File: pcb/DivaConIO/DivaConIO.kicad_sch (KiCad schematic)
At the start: 59 parts, among them J1 Conn_01x06_MountingPin, J2 Conn_01x04_MountingPin, J3 Conn_01x06_MountingPin, J4 Conn_01x08_MountingPin, J5 JST_SH_BM03B-SRSS-TB, J6 Conn_01x05_MountingPin, J7 Conn_01x06_MountingPin, Q1 BSS138, Q2 BSS138, Q3 BSS138, Q4 BSS138, Q5 BSS138, SW1 SW_Push

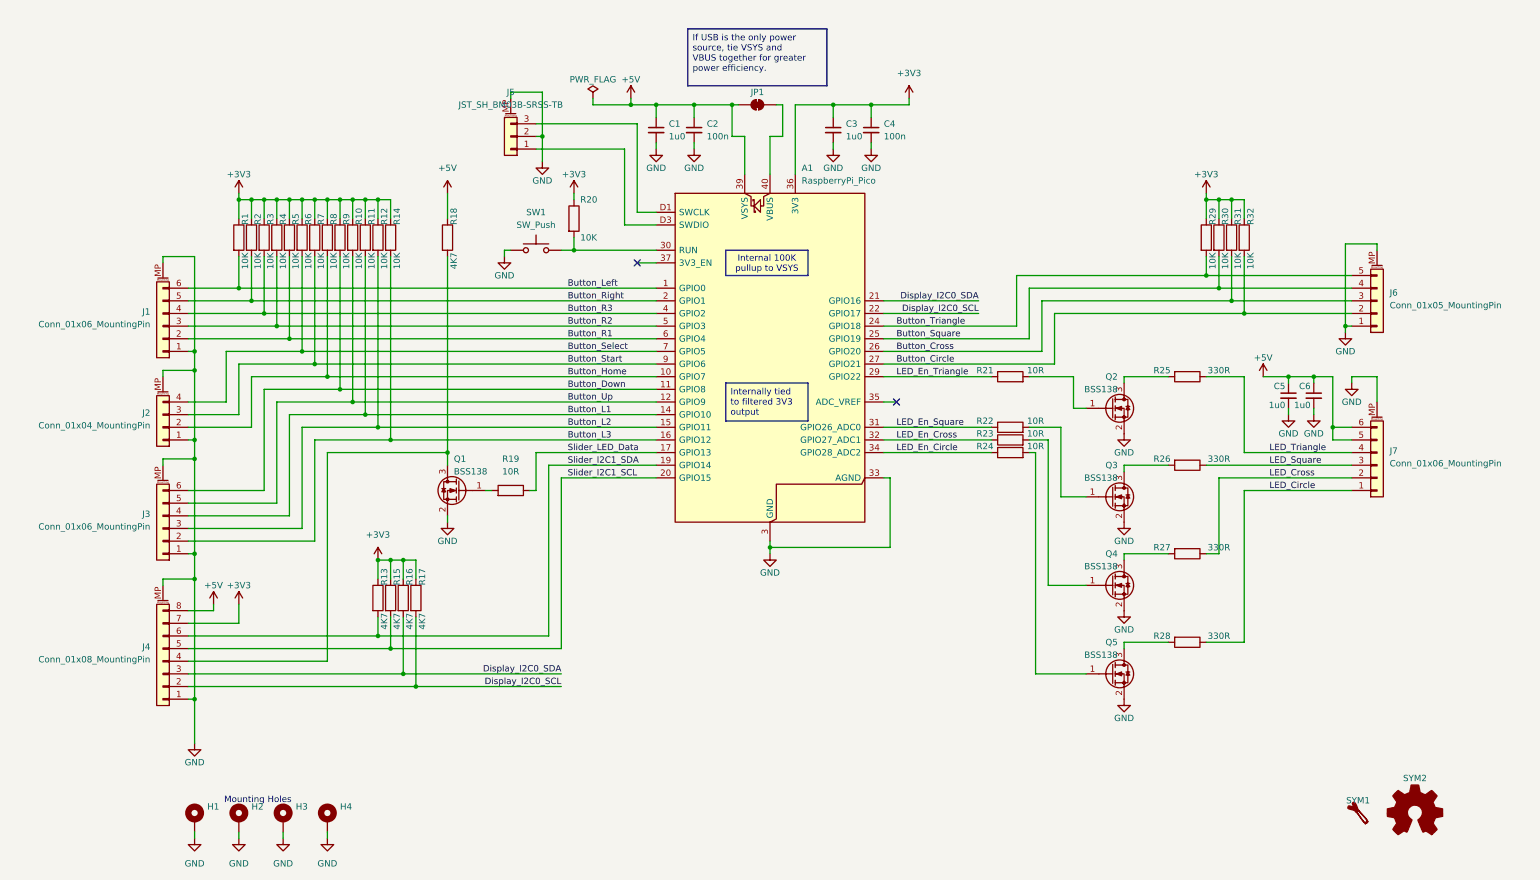
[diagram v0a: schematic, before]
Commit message: revision 1.0 pcb schematics and layout
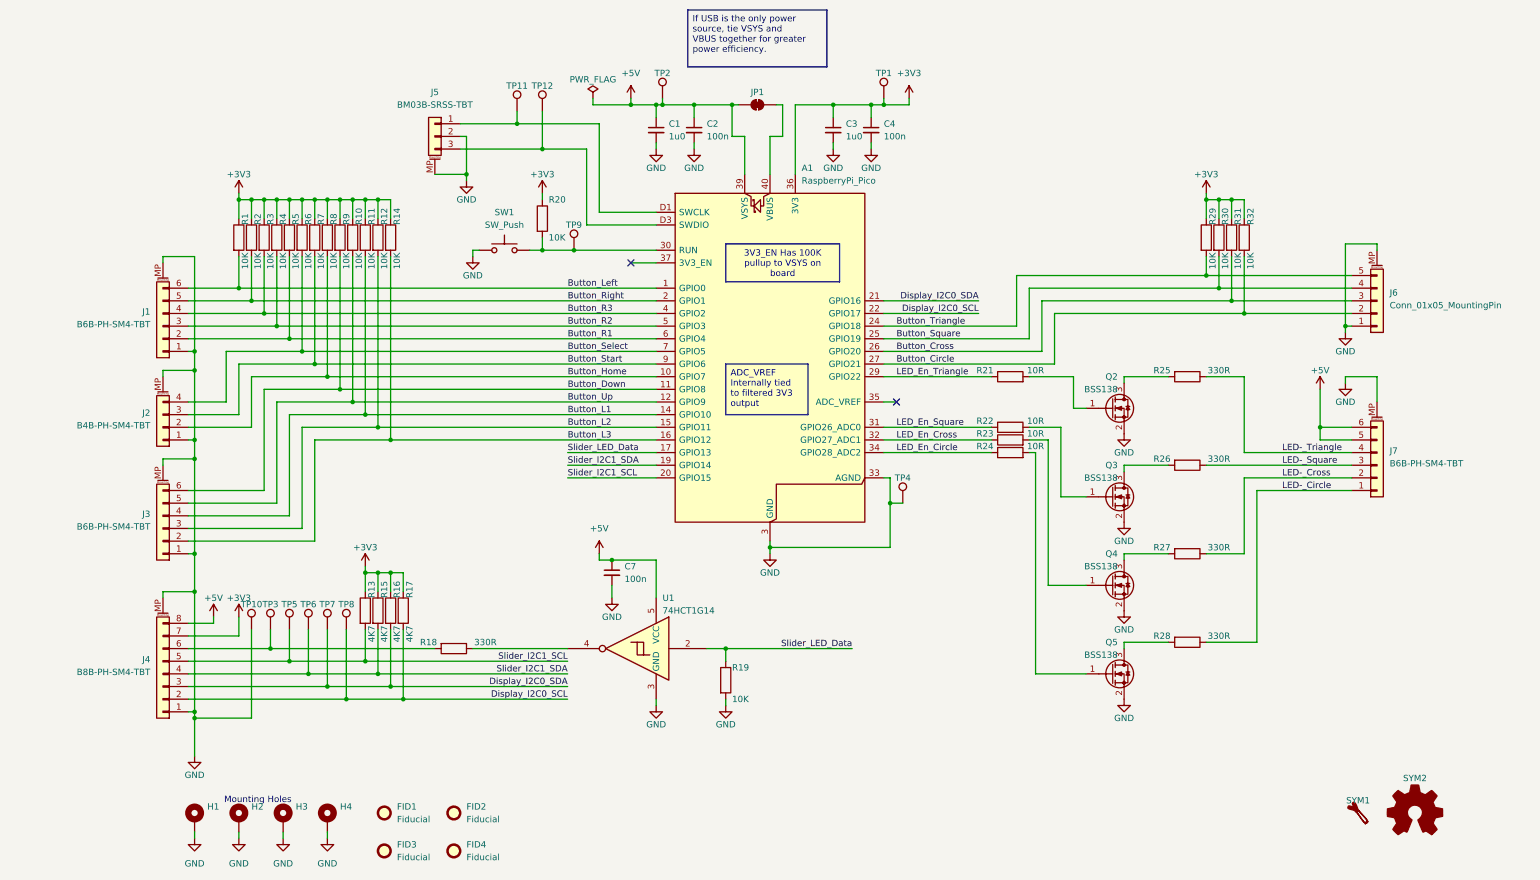
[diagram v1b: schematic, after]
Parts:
- removed C5, C6: 1u0, Capacitor_SMD:C_0603_1608Metric, symbol Device:C_Small
- removed Q1: BSS138, Package_TO_SOT_SMD:SOT-23, symbol Transistor_FET:BSS138
- added C7: 100n, Capacitor_SMD:C_0603_1608Metric, symbol Device:C_Small
- added FID1, FID2, FID3, FID4: Fiducial, Fiducial:Fiducial_0.5mm_Mask1.5mm, symbol Mechanical:Fiducial
- added TP1, TP10, TP11, TP12, TP2, TP3, TP4, TP5, TP6, TP7, TP8, TP9: TestPoint, TestPoint:TestPoint_Pad_D2.0mm, symbol Connector:TestPoint
- added U1: 74HCT1G14, Package_TO_SOT_SMD:SC-74A-5_1.55x2.9mm_P0.95mm, symbol 74xGxx:74AHCT1G14
- J1, J3, J7: value Conn_01x06_MountingPin -> B6B-PH-SM4-TBT
- J2: value Conn_01x04_MountingPin -> B4B-PH-SM4-TBT
- J4: value Conn_01x08_MountingPin -> B8B-PH-SM4-TBT
- J5: value JST_SH_BM03B-SRSS-TB -> BM03B-SRSS-TBT
- R18: value 4K7 -> 330R
- R19: value 10R -> 10K
- SW1: footprint Button_Switch_SMD:SW_Push_SPST_NO_Alps_SKRK -> DivaConIO:SW_Push_SPST_NO_Alps_SKRP
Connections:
- net +3V3: now also TP1.1
- net +5V: now also C7.1, TP2.1, U1.5 (VCC); no longer R18.1
- net Display_I2C0_SCL: now also TP8.1
- net Display_I2C0_SDA: now also TP7.1
- net GND: now also R19.2, C7.2, TP10.1, TP4.1, U1.3 (GND)
- net Slider_I2C1_SCL: now also R13.2, TP5.1; no longer R15.2
- net Slider_I2C1_SDA: now also J4.4 (Pin_4), R15.2, TP6.1; no longer J4.6 (Pin_6), R13.2
- net Slider_LED_Data: now also U1.2
- net at R18.2: now also J4.6 (Pin_6), TP3.1; no longer J4.4 (Pin_4)
- net at J5.1 (Pin_1): now also A1.D1 (SWCLK), TP11.1; no longer A1.D3 (SWDIO)
- net at J5.3 (Pin_3): now also A1.D3 (SWDIO), TP12.1; no longer A1.D1 (SWCLK)
- net at A1.30 (RUN), R20.2, SW1.2: now also TP9.1
- net LED_Circle renamed LED-_Circle
- net LED_Cross renamed LED-_Cross
- net LED_Square renamed LED-_Square
- net LED_Triangle renamed LED-_Triangle
- new net: R18.1, U1.4
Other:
- moved on the sheet: J4, J5, R13, R15, R16, R17, R20, SW1

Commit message: revision 1.1 pcb schematics and layout
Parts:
- removed R23: 10R, Resistor_SMD:R_0603_1608Metric, symbol Device:R
- removed R26: 330R, Resistor_SMD:R_0603_1608Metric, symbol Device:R
- added R20: 10R, Resistor_SMD:R_0603_1608Metric, symbol Device:R
- added R32: 330R, Resistor_SMD:R_0603_1608Metric, symbol Device:R
- renumbered C7 to C5, FID3 to FID2, FID2 to FID3, J6 to J4, J4 to J6, Q5 to Q1, Q4 to Q2, Q2 to Q4, R9 to R10, R31 to R11, R10 to R12, R30 to R13, R11 to R14, R29 to R15, R12 to R16, R14 to R17, R20 to R18, R24 to R19, R19 to R23, R28 to R24, R18 to R26, R17 to R28, R16 to R29, R15 to R30, R13 to R31, R32 to R9, TP12 to TP1, TP5 to TP10, TP3 to TP11, TP10 to TP12, TP11 to TP2, TP9 to TP3, TP2 to TP4, TP4 to TP5, TP1 to TP6, TP8 to TP7, TP7 to TP8, TP6 to TP9
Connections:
- net +3V3: now also J6.5 (Pin_5), TP5.1; no longer J6.7 (Pin_7), TP6.1
- net +5V: now also J6.7 (Pin_7), J7.1 (Pin_1), J7.2 (Pin_2); no longer J6.8 (Pin_8), J7.5 (Pin_5), J7.6 (Pin_6)
- net Button_Circle: now also A1.17 (GPIO13), J4.5 (Pin_5); no longer A1.27 (GPIO21), J4.2 (Pin_2)
- net Button_Cross: now also A1.19 (GPIO14), J4.4 (Pin_4); no longer A1.26 (GPIO20), J4.3 (Pin_3)
- net Button_Square: now also A1.20 (GPIO15), J4.3 (Pin_3); no longer A1.25 (GPIO19), J4.4 (Pin_4)
- net Button_Triangle: now also A1.21 (GPIO16), J4.2 (Pin_2); no longer A1.24 (GPIO18), J4.5 (Pin_5)
- net Display_I2C0_SCL: now also A1.27 (GPIO21), J6.1 (Pin_1), R31.2, TP11.1; no longer A1.22 (GPIO17), J6.2 (Pin_2), R28.2, TP7.1
- net Display_I2C0_SDA: now also A1.26 (GPIO20), J6.2 (Pin_2), R30.2, TP10.1; no longer A1.21 (GPIO16), J6.3 (Pin_3), R29.2, TP8.1
- net GND: now also J6.6 (Pin_6), TP6.1; no longer J6.1 (Pin_1), TP5.1
- net LED-_Circle: now also J7.6 (Pin_6), R32.1; no longer J7.1 (Pin_1), R24.1
- net LED-_Cross: now also J7.5 (Pin_5); no longer J7.2 (Pin_2)
- net LED-_Square: now also J7.4 (Pin_4), R25.1; no longer J7.3 (Pin_3)
- net LED-_Triangle: now also J7.3 (Pin_3), R24.1; no longer J7.4 (Pin_4), R25.1
- net LED_En_Circle: now also A1.29 (GPIO22), R22.1; no longer A1.34 (GPIO28_ADC2), R19.1
- net LED_En_Cross: now also A1.31 (GPIO26_ADC0), R21.1; no longer A1.32 (GPIO27_ADC1)
- net LED_En_Square: now also A1.32 (GPIO27_ADC1), R20.1; no longer A1.31 (GPIO26_ADC0), R22.1
- net LED_En_Triangle: now also A1.34 (GPIO28_ADC2), R19.1; no longer A1.29 (GPIO22), R21.1
- net Slider_I2C1_SCL: now also A1.25 (GPIO19), J6.3 (Pin_3), R29.2, TP9.1; no longer A1.20 (GPIO15), J6.5 (Pin_5), R31.2, TP10.1
- net Slider_I2C1_SDA: now also A1.24 (GPIO18), R28.2, TP8.1; no longer A1.19 (GPIO14), R30.2, TP9.1
- net Slider_LED_Data: now also A1.22 (GPIO17); no longer A1.17 (GPIO13)
- net at Q2.1 (G): now also R20.2
- net at Q2.3 (D): now also R25.2; no longer R27.2
- net at R22.2: now also Q4.1 (G); no longer Q3.1 (G)
- net at Q3.3 (D): now also R27.2
- net at R21.2: now also Q3.1 (G); no longer Q4.1 (G)
- net at Q4.3 (D): now also R32.2; no longer R25.2
- net at A1.D1 (SWCLK), J5.1 (Pin_1): now also TP1.1; no longer TP2.1
- net at A1.D3 (SWDIO), J5.3 (Pin_3): now also TP2.1; no longer TP1.1
- new net: J6.8 (Pin_8), R26.2, TP7.1
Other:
- moved on the sheet: A1, C1, C2, C3, C4, C5, FID1, FID2, FID3, FID4, H1, H2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
